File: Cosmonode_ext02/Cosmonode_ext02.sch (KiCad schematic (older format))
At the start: 22 parts, among them J1 CONN_01X04, J2 CONN_01X04, J3 CONN_01X12, J4 CONN_01X12, J5 GS3, J6 GS3, J7 Aloes_Logo, J8 OSHW_Logo, J9 CONN_01X04, Q1 BSS138, Q2 BSS138, SW1 SW_Push, SW2 SW_Push, U1 XC6206P502MR

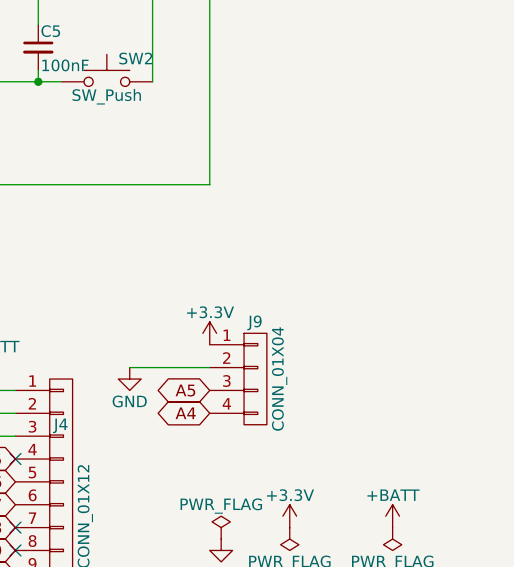
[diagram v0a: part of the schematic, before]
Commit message: fix and update
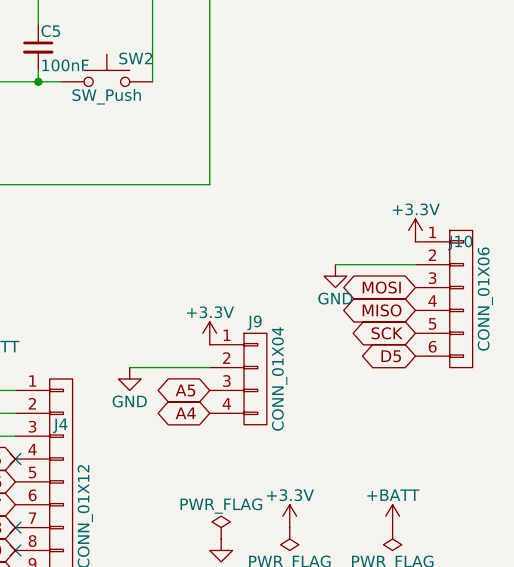
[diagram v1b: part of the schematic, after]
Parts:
- added J10: CONN_01X06, Pin_Headers:Pin_Header_Straight_1x06_Pitch2.54mm, symbol CONN_01X06
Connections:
- net +3V3: now also J10.1 (P1)
- net D5: now also J10.6 (P6)
- net GND: now also J10.2 (P2)
- net MISO: now also J10.4 (P4)
- net MOSI: now also J10.3 (P3)
- net SCK: now also J10.5 (P5)
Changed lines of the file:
@@
 Text GLabel 7250 4800 0    51   BiDi ~ 0
 A4
+$Comp
+L CONN_01X06 J10
+U 1 1 5A34520B
+P 10150 4100
+F 0 "J10" H 10150 4350 50  0000 C CNN
+F 1 "CONN_01X06" V 10250 4100 50  0000 C CNN
+F 2 "Pin_Headers:Pin_Header_Straight_1x06_Pitch2.54mm" H 10150 4100 50  0001 C CNN
+F 3 "" H 10150 4100 50  0001 C CNN
+	1    10150 4100
+	1    0    0    -1
+$EndComp
+$Comp
+L +3.3V #PWR019
+U 1 1 5A345213
+P 9950 3850
+F 0 "#PWR019" H 9950 3700 50  0001 C CNN
+F 1 "+3.3V" H 9950 3990 50  0000 C CNN
+F 2 "" H 9950 3850 50  0001 C CNN
+F 3 "" H 9950 3850 50  0001 C CNN
+	1    9950 3850
+	1    0    0    -1
+$EndComp
+$Comp
+L GND #PWR020
+U 1 1 5A345219
+P 9600 3950
+F 0 "#PWR020" H 9600 3700 50  0001 C CNN
+F 1 "GND" H 9600 3800 50  0000 C CNN
+F 2 "" H 9600 3950 50  0001 C CNN
+F 3 "" H 9600 3950 50  0001 C CNN
+	1    9600 3950
+	1    0    0    -1
+$EndComp
+Wire Wire Line
+	9950 3950 9600 3950
+Text GLabel 9950 4350 0    51   BiDi ~ 0
+D5
+Text GLabel 9950 4050 0    51   BiDi ~ 0
+MOSI
+Text GLabel 9950 4150 0    51   BiDi ~ 0
+MISO
+Text GLabel 9950 4250 0    51   BiDi ~ 0
+SCK
 $EndSCHEMATC
